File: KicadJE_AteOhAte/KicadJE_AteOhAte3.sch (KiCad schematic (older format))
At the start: 86 parts, among them J301 PJRAS2X2S01AUX, J302 Conn_01x03, U301 TL072, U302 TL072, U303 TL072

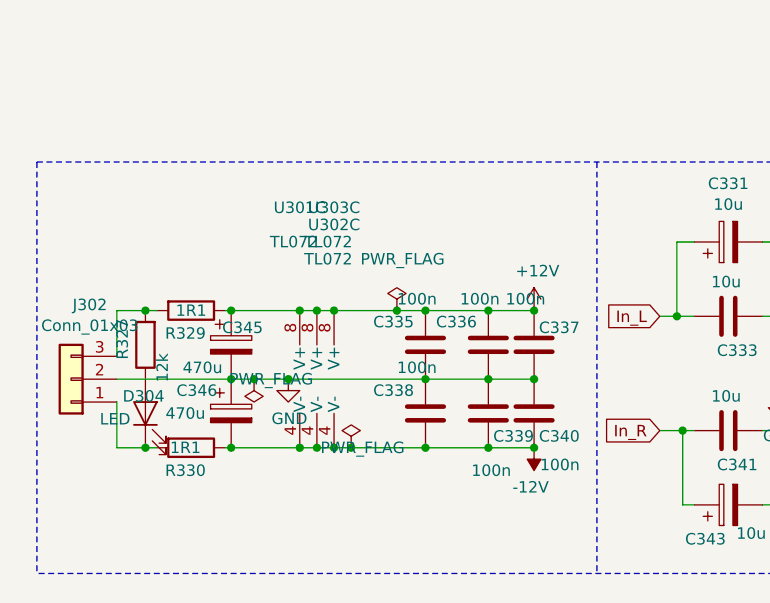
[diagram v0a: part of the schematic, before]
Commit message: Fused RIAA SCH
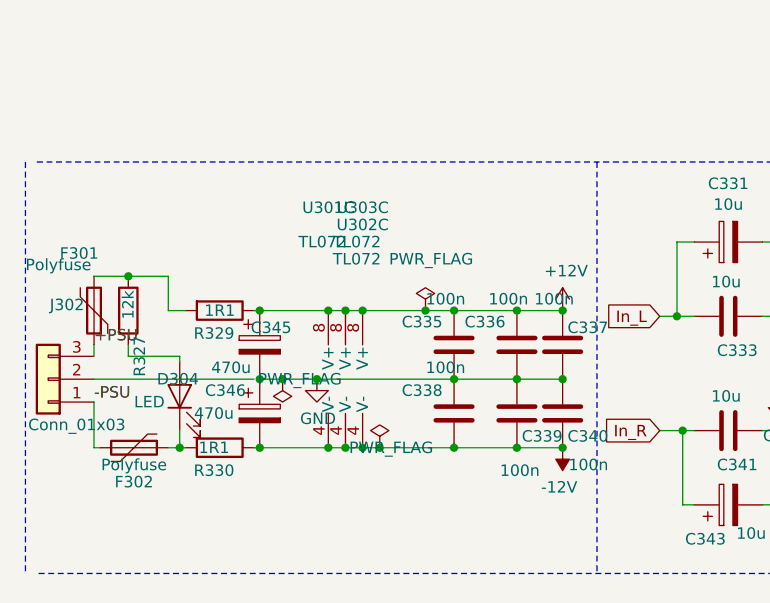
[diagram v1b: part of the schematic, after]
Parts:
- added F301, F302: Polyfuse, Fuse:Fuse_1206_3216Metric, symbol Device:Polyfuse
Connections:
- net GND: no longer J302.2 (Pin_2)
- net at D304.1 (K), R330.2: now also F302.1; no longer J302.1 (Pin_1)
- net at D304.2 (A): now also R327.2; no longer R327.1
- new net: F301.2, R327.1, R329.2
- new net +PSU: F301.1, J302.3 (Pin_3)
- new net -PSU: F302.2, J302.1 (Pin_1)
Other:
- moved on the sheet: C335, C336, C337, C338, C339, C340, C345, C346, D304, J302, R327, R329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
